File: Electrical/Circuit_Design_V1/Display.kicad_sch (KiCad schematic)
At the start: 1 part

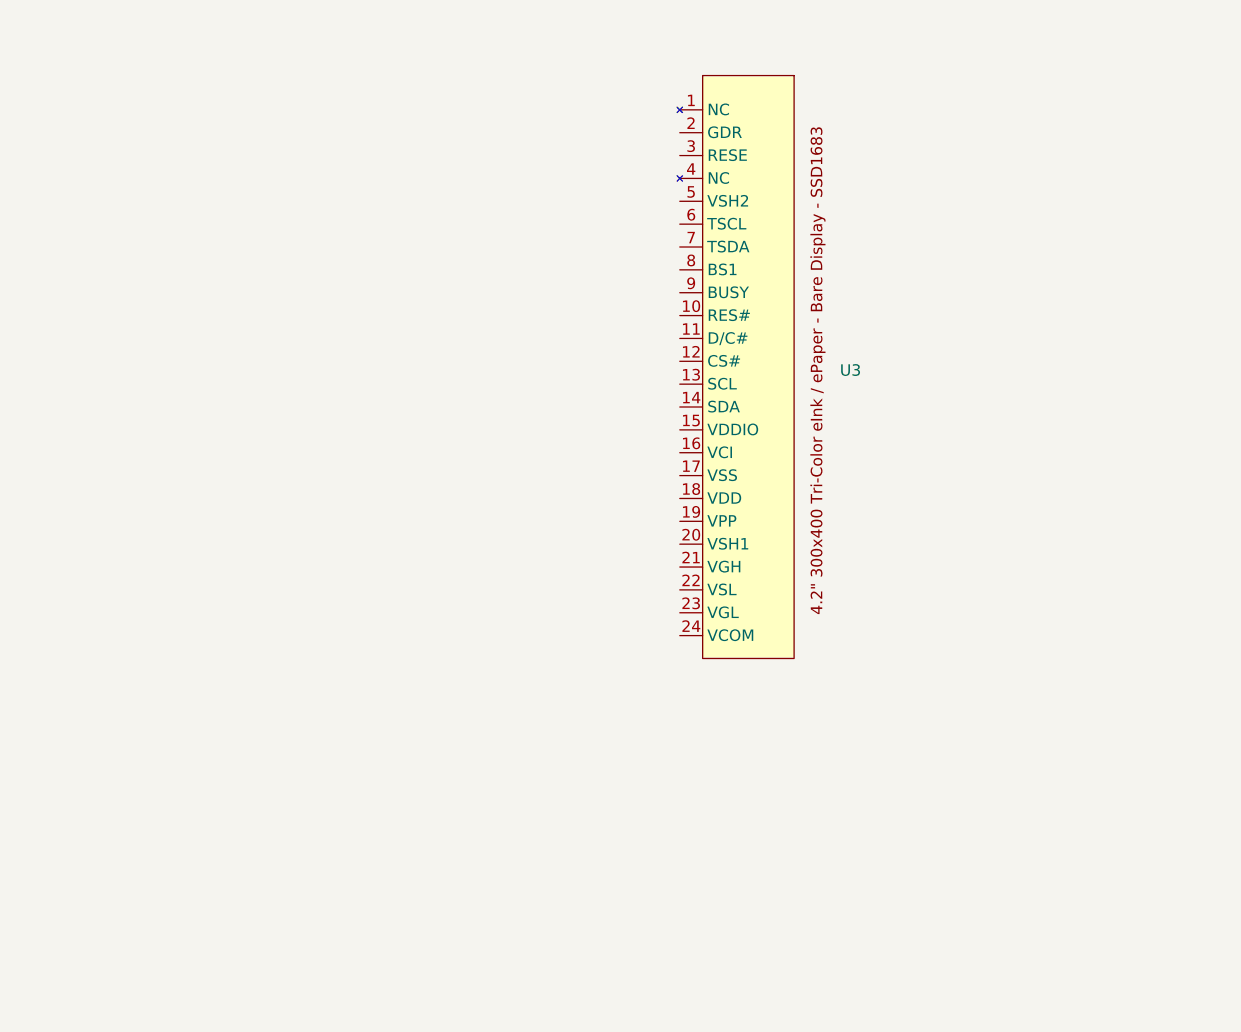
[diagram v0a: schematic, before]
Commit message: #3 Finishing some circuitry.
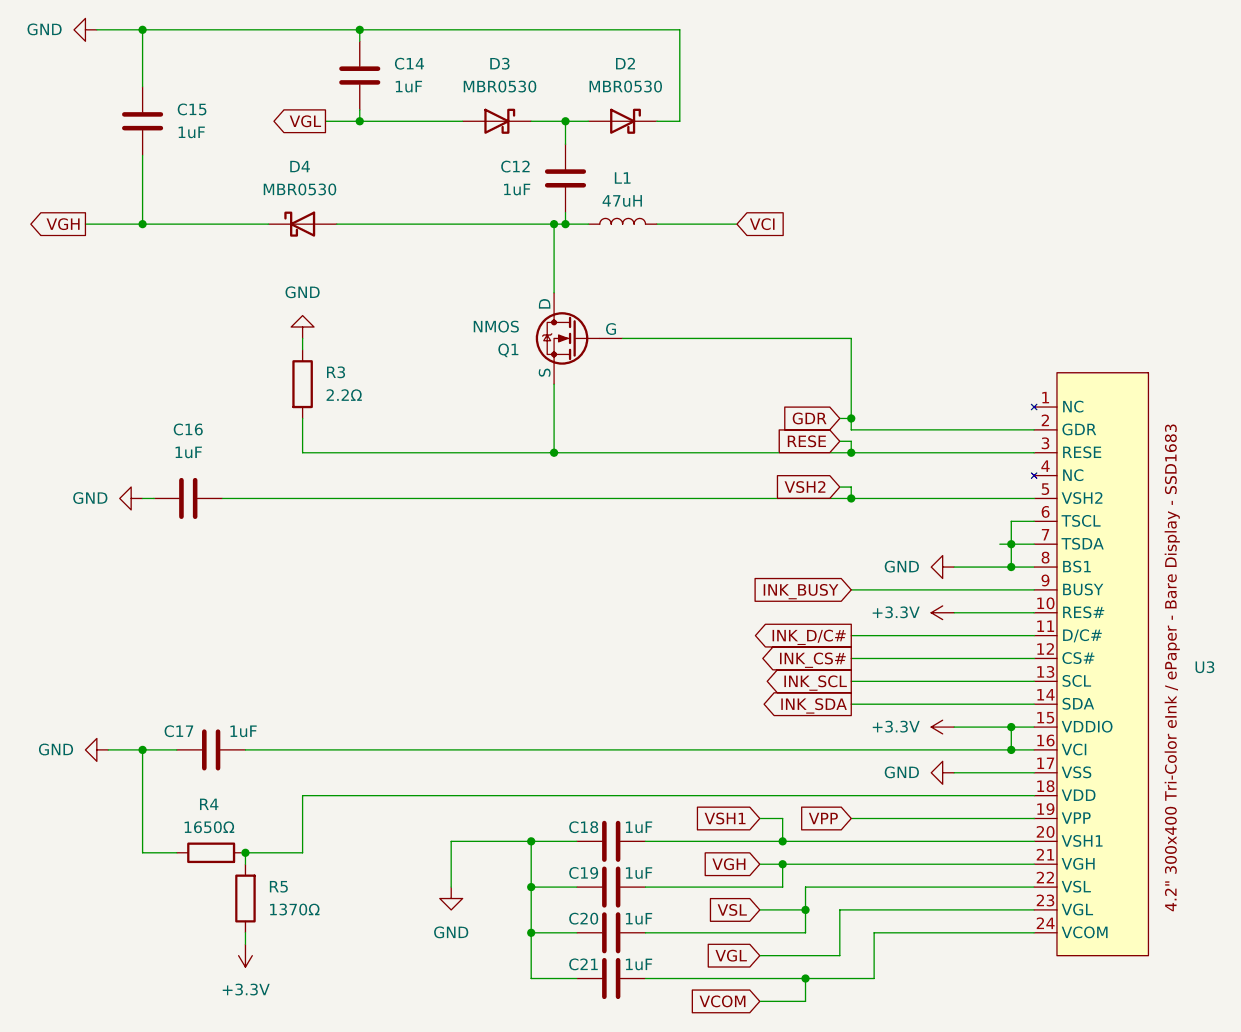
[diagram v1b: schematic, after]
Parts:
- added C12, C14, C15, C16, C17, C18, C19, C20, C21: 1uF, Capacitor_SMD:C_0805_2012Metric, symbol Device:C
- added D2, D3, D4: MBR0530, Diode_SMD:D_SOD-123, symbol Diode:MBR0530
- added L1: 47uH, Etchasketch_Footprints:Inductor, symbol Device:L
- added Q1: NMOS, Package_TO_SOT_SMD:TSOT-23, symbol Simulation_SPICE:NMOS
- added R3: 2.2Ω, Resistor_SMD:R_0805_2012Metric_Pad1.20x1.40mm_HandSolder, symbol Device:R
- added R4: 1650Ω, Resistor_SMD:R_0805_2012Metric, symbol Device:R
- added R5: 1370Ω, Resistor_SMD:R_0805_2012Metric, symbol Device:R
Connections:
- net +3.3V: now reaches U3.10 (RES#)
- net +3.3V: now also U3.15 (VDDIO), U3.16 (VCI), C17.2, R5.1
- net INK_D/C#: now reaches U3.11 (D/C#)
- net INK_CS#: now reaches U3.12 (CS#)
- net INK_SCL: now reaches U3.13 (SCL)
- net INK_SDA: now reaches U3.14 (SDA)
- net GND: now reaches U3.17 (VSS)
- net GND: now also U3.6 (TSCL), U3.7 (TSDA), U3.8 (BS1), C14.1, C15.1, C16.1, C17.1, C18.1, C19.1, C20.1, C21.1, D2.1 (K), R3.1, R4.1
- net at U3.18 (VDD): now also R4.2, R5.2
- net VPP: now reaches U3.19 (VPP)
- net GDR: now reaches U3.2 (GDR)
- net GDR: now also Q1.2 (G)
- net VSH1: now reaches U3.20 (VSH1)
- net VSH1: now also C18.2
- net VGH: now reaches U3.21 (VGH)
- net VGH: now also C15.2, C19.2, D4.1 (K)
- net VSL: now reaches U3.22 (VSL)
- net VSL: now also C20.2
- net VGL: now reaches U3.23 (VGL)
- net VGL: now also C14.2, D3.2 (A)
- net VCOM: now reaches U3.24 (VCOM)
- net VCOM: now also C21.2
- net RESE: now reaches U3.3 (RESE)
- net RESE: now also Q1.3 (S), R3.2
- net VSH2: now reaches U3.5 (VSH2)
- net VSH2: now also C16.2
- net INK_BUSY: now reaches U3.9 (BUSY)
- new net: C12.1, D2.2 (A), D3.1 (K)
- new net: C12.2, D4.2 (A), L1.1, Q1.1 (D)
- new net VCI: L1.2
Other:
- moved on the sheet: U3
